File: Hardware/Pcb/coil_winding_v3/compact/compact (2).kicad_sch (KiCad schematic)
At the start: 25 parts, among them J1 Conn_01x14_Pin, J2 Screw_Terminal_01x02, J3 Conn_01x03_Socket, J4 Conn_01x03_Socket, M1 Motor_DC, Q3 IRFZ40, SW1 SW_SPST, SW2 SW_SPST, SW3 RotaryEncoder_Switch, U1 LM7805_TO220

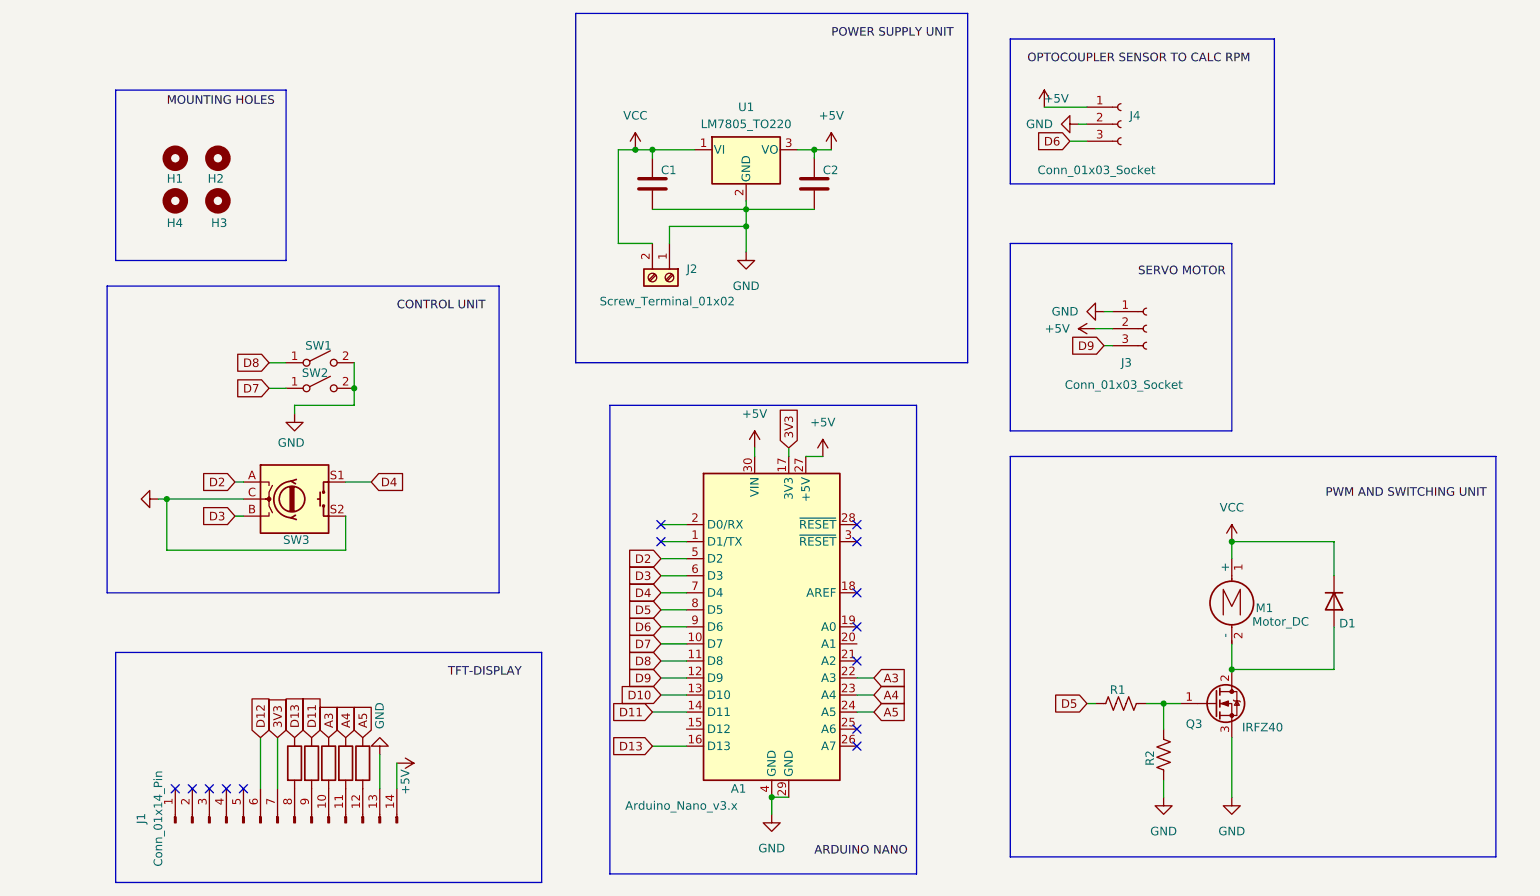
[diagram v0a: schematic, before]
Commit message: tuesday
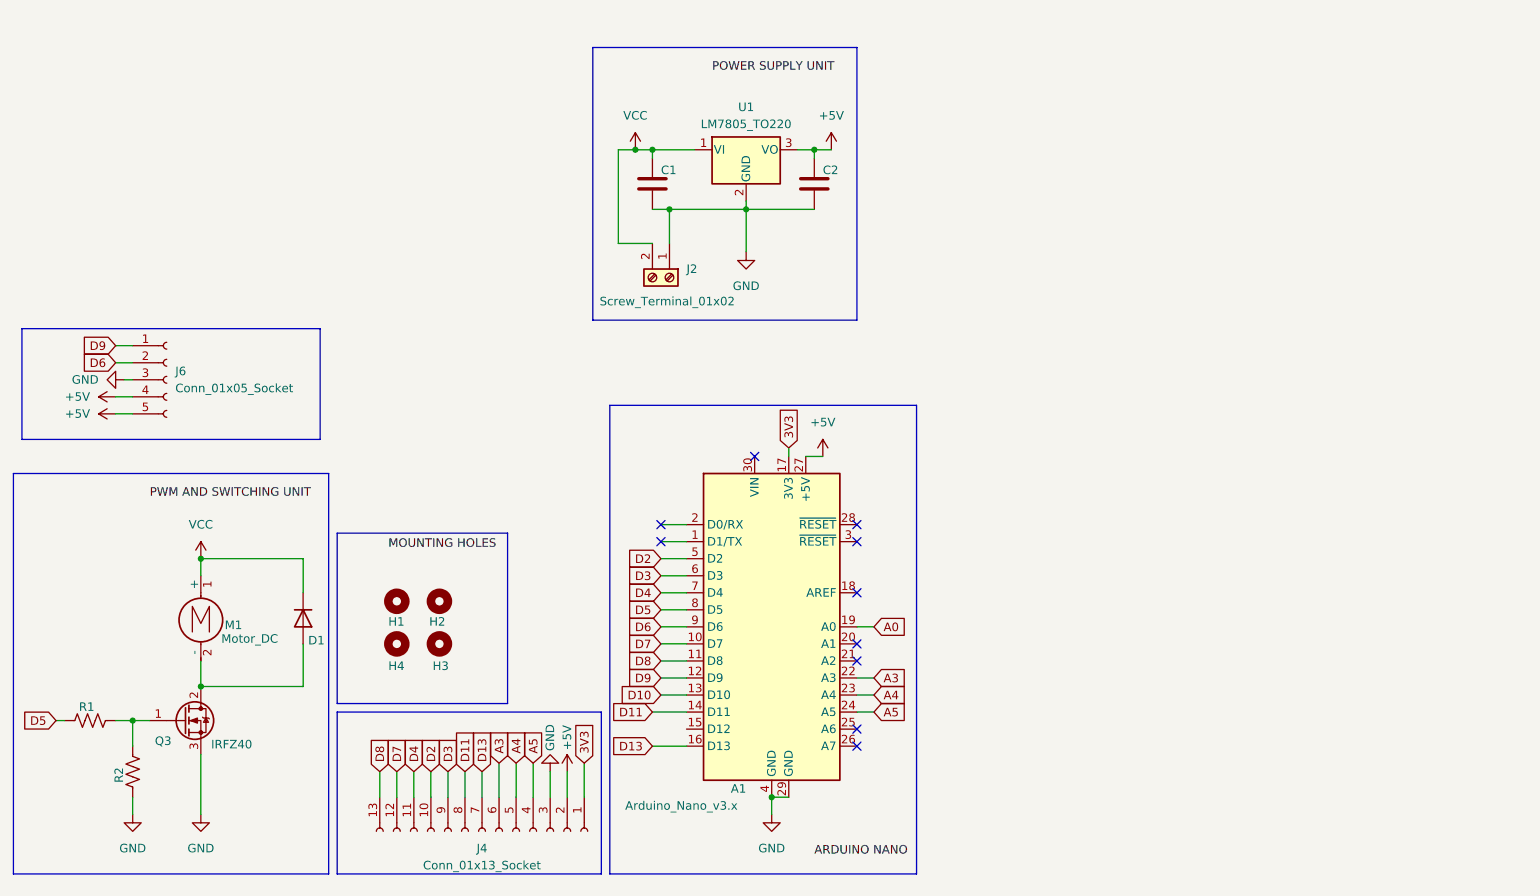
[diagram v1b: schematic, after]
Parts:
- removed J1: Conn_01x14_Pin, Connector_PinSocket_2.54mm:PinSocket_1x14_P2.54mm_Vertical, symbol Connector:Conn_01x14_Pin
- removed J3: Conn_01x03_Socket, Connector_PinSocket_2.54mm:PinSocket_1x03_P2.54mm_Vertical, symbol Connector:Conn_01x03_Socket
- removed J4: Conn_01x03_Socket, Connector_PinHeader_2.54mm:PinHeader_1x03_P2.54mm_Vertical, symbol Connector:Conn_01x03_Socket
- removed R10, R11, R12, R13, R9: R, Resistor_THT:R_Axial_DIN0207_L6.3mm_D2.5mm_P7.62mm_Horizontal, symbol Device:R
- removed SW1, SW2: SW_SPST, Button_Switch_THT:SW_PUSH_6mm_H7.3mm, symbol Switch:SW_SPST
- removed SW3: RotaryEncoder_Switch, Rotary_Encoder:RotaryEncoder_Alps_EC12E-Switch_Vertical_H20mm, symbol Device:RotaryEncoder_Switch
- added J4: Conn_01x13_Socket, Connector_PinHeader_2.54mm:PinHeader_2x13_P2.54mm_Vertical, symbol Connector:Conn_01x13_Socket
- added J6: Conn_01x05_Socket, Connector_PinHeader_2.54mm:PinHeader_2x05_P2.54mm_Vertical, symbol Connector:Conn_01x05_Socket
- M1: footprint Connector_PinHeader_2.54mm:PinHeader_1x02_P2.54mm_Vertical -> TerminalBlock:TerminalBlock_Xinya_XY308-2.54-2P_1x02_P2.54mm_Horizontal
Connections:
- net +5V: now also J4.2 (Pin_2), J6.4 (Pin_4), J6.5 (Pin_5); no longer A1.30 (VIN)
- net 3V3: now also J4.1 (Pin_1)
- net A3: now also J4.6 (Pin_6)
- net A4: now also J4.5 (Pin_5)
- net A5: now also J4.4 (Pin_4)
- net D11: now also J4.8 (Pin_8)
- net D13: now also J4.7 (Pin_7)
- net D2: now also J4.10 (Pin_10)
- net D3: now also J4.9 (Pin_9)
- net D4: now also J4.11 (Pin_11)
- net D6: now also J6.2 (Pin_2)
- net D7: now also J4.12 (Pin_12)
- net D8: now also J4.13 (Pin_13)
- net D9: now also J6.1 (Pin_1)
- net GND: now also J4.3 (Pin_3), J6.3 (Pin_3)
- net A0: now reaches A1.19 (A0)
- no-connect marks 14 -> 10
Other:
- moved on the sheet: D1, H1, H2, H3, H4, M1, Q3, R1, R2

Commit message: final_code
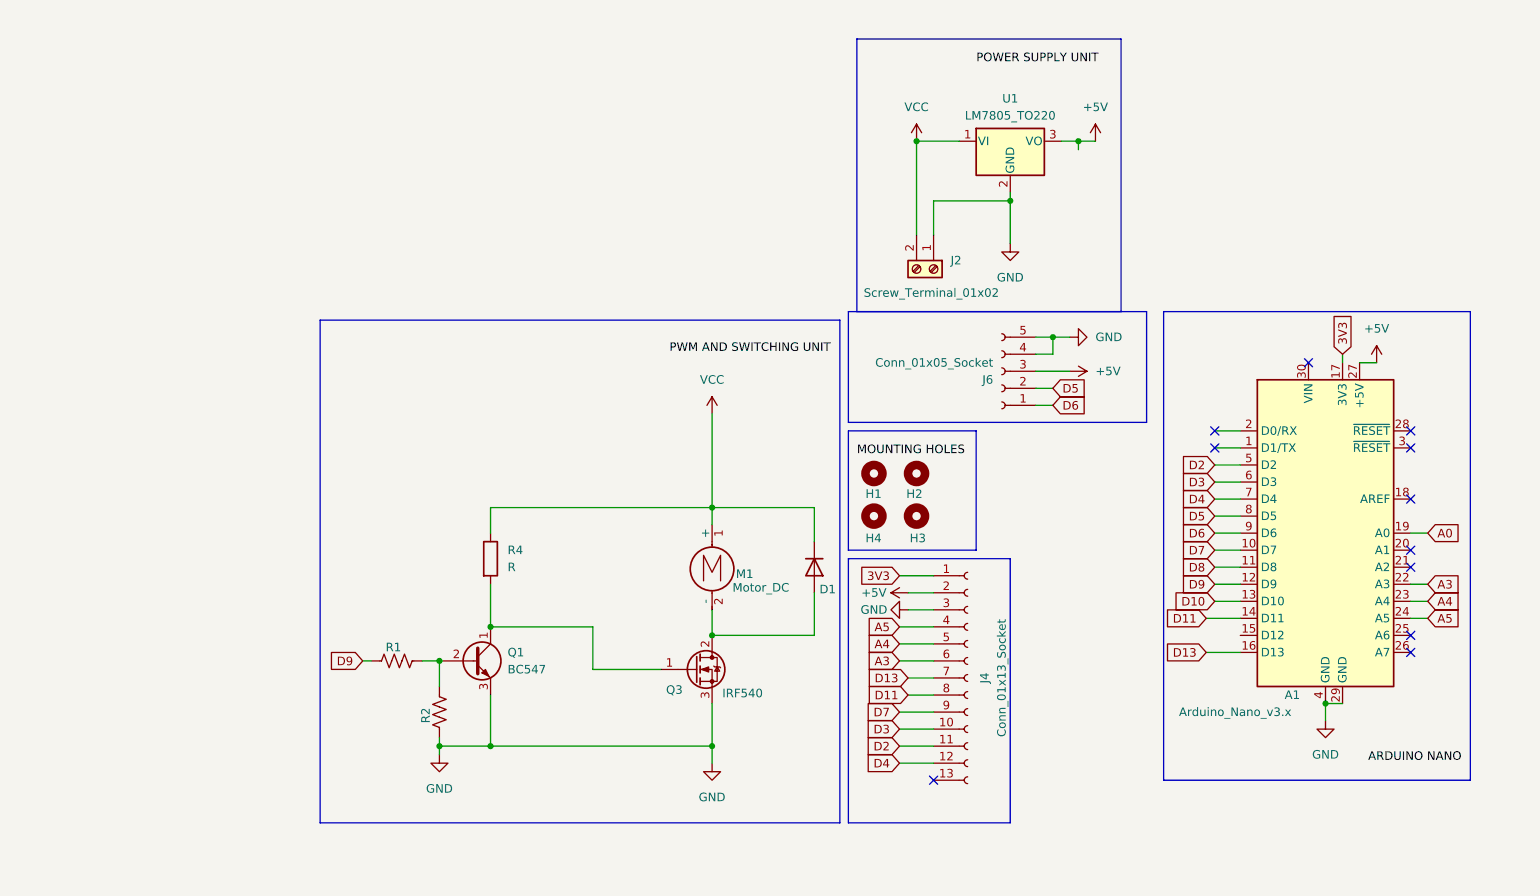
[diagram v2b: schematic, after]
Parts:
- removed C1, C2: C, Capacitor_THT:CP_Radial_D5.0mm_P2.00mm, symbol Device:C
- added Q1: BC547, Package_TO_SOT_THT:TO-92_Inline, symbol Transistor_BJT:BC547
- added R4: R, Resistor_THT:R_Axial_DIN0207_L6.3mm_D2.5mm_P7.62mm_Horizontal, symbol Device:R
- J2: footprint Connector_BarrelJack:BarrelJack_Horizontal -> TerminalBlock_4Ucon:TerminalBlock_4Ucon_1x02_P3.50mm_Horizontal
- M1: footprint TerminalBlock:TerminalBlock_Xinya_XY308-2.54-2P_1x02_P2.54mm_Horizontal -> TerminalBlock_4Ucon:TerminalBlock_4Ucon_1x02_P3.50mm_Horizontal
- Q3: value IRFZ40 -> IRF540
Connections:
- net +5V: now also J6.3 (Pin_3); no longer J6.4 (Pin_4), J6.5 (Pin_5)
- net D2: now also J4.11 (Pin_11); no longer J4.10 (Pin_10)
- net D3: now also J4.10 (Pin_10); no longer J4.9 (Pin_9)
- net D4: now also J4.12 (Pin_12); no longer J4.11 (Pin_11)
- net D5: now also J6.2 (Pin_2); no longer R1.1
- net D6: now also J6.1 (Pin_1); no longer J6.2 (Pin_2)
- net D7: now also J4.9 (Pin_9); no longer J4.12 (Pin_12)
- net D8: no longer J4.13 (Pin_13)
- net D9: now also R1.1; no longer J6.1 (Pin_1)
- net GND: now also J6.4 (Pin_4), J6.5 (Pin_5), Q1.3 (E); no longer J6.3 (Pin_3)
- net VCC: now also R4.1
- net at R1.2, R2.2: now also Q1.2 (B); no longer Q3.1 (G)
- new net: Q1.1 (C), Q3.1 (G), R4.2
- no-connect marks 10 -> 11
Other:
- moved on the sheet: A1, D1, H1, H2, H3, H4, J2, J4, J6, M1, Q3, R1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
